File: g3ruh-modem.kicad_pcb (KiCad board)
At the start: 2 copper layers, 160 x 100 mm, 112 parts, among them P1 CONN_01X03, P2 CONN_01X06, P3 CONN_01X05, P4 C96ABC, Q1 LM7805_TO220, U1 4029, U10 LM339, U11 74HC14, U12 74HC164, U13 74HC86, U14 74HC164, U15 27C128, U16 TL084, U17 74HC74, U18 74HC164, U19 ZN429E-8, U2 27C128, U3 4029, U4 74HC164, U5 74HC74, U6 74HC86, U7 74HC164, U8 74HC161, U9 ZN429E-8

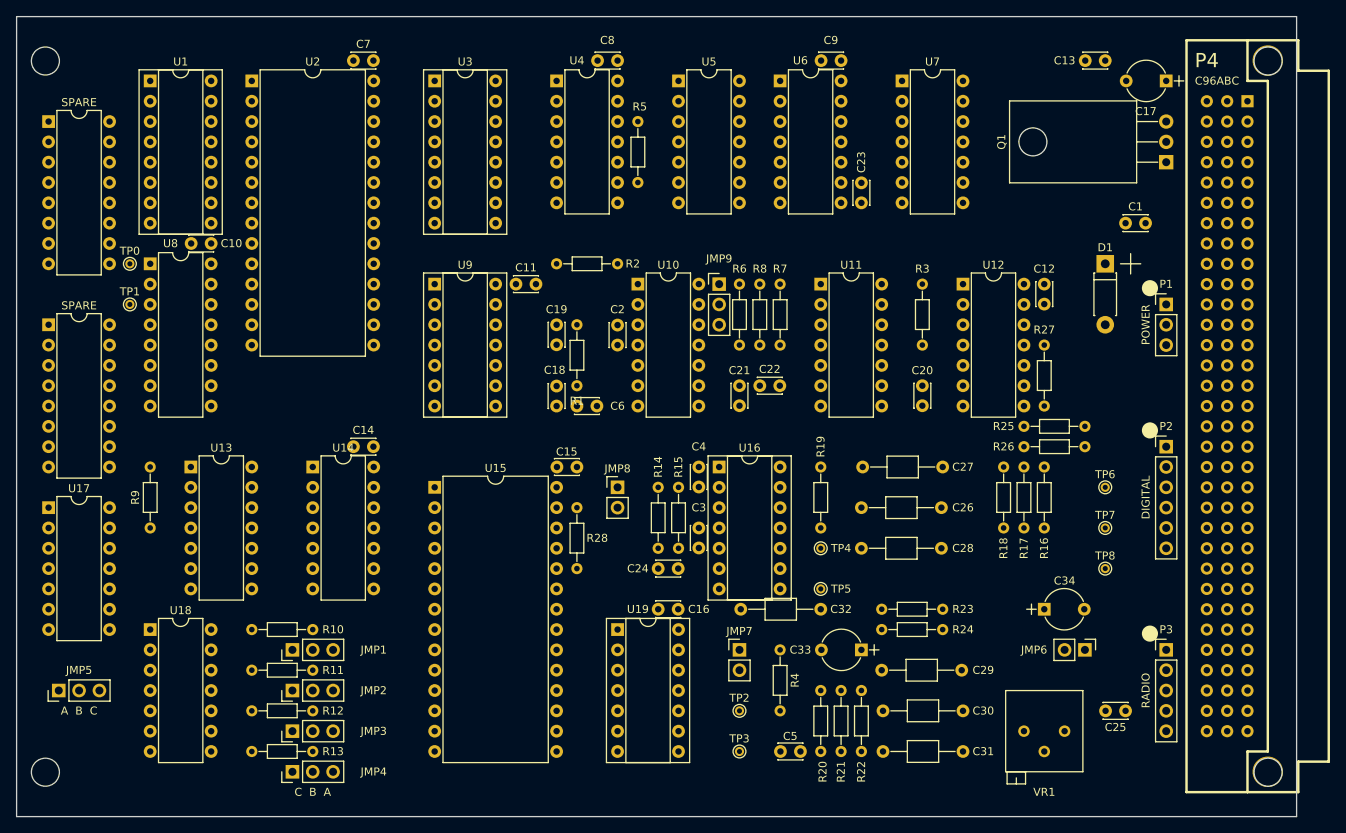
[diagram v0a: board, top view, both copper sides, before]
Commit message: Completed routing.
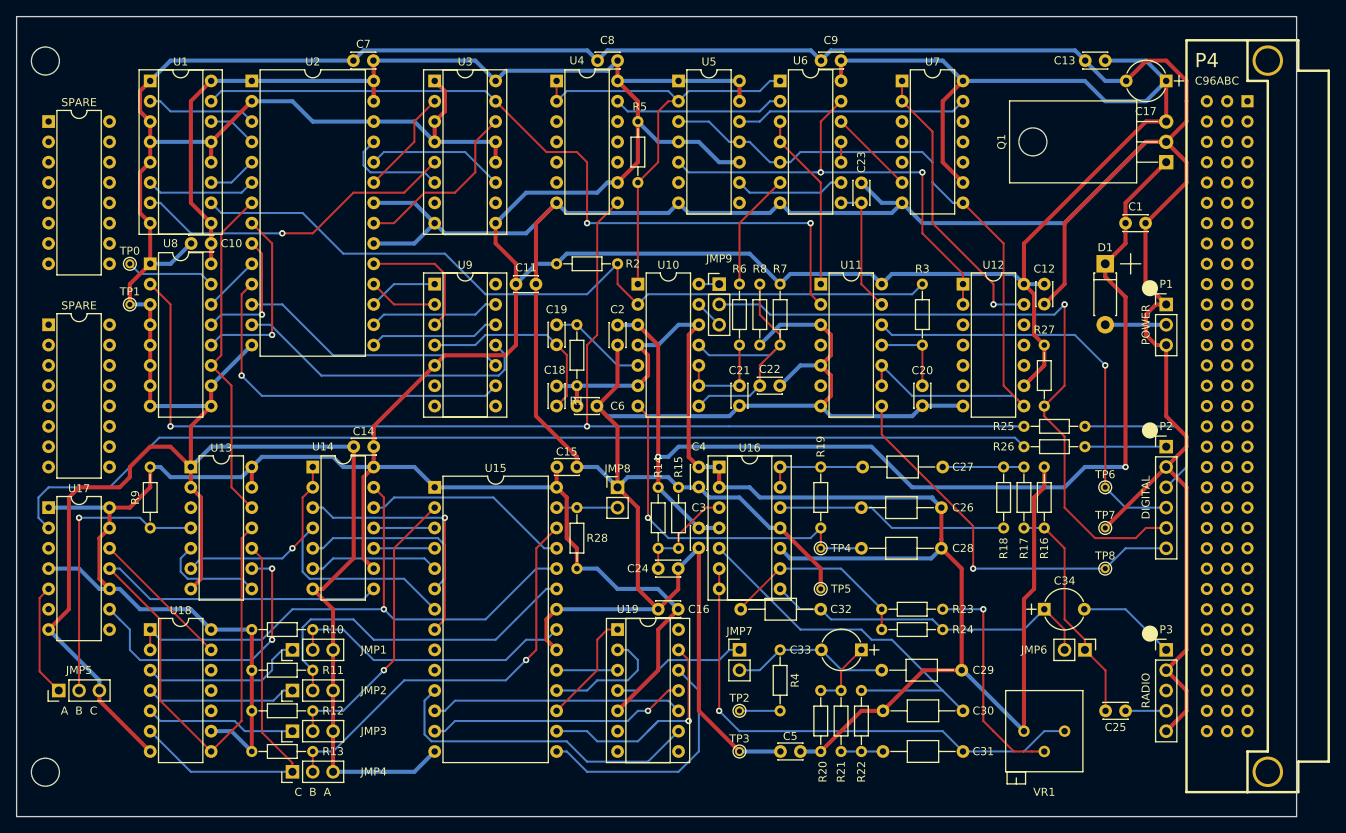
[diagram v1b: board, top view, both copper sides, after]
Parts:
- removed the REF** at (229.6, 137.8)
- removed the REF** at (229.6, 48.9)
- moved C14 2.54 mm to (117.8, 97.1), turned to 180 degrees
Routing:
- net GND: track 0.00 -> 940.6 mm
- net +5V: track 0.00 -> 575.9 mm
- net VREF: track 0.00 -> 192.3 mm
- net /ZERO CROSSING/TX_CLOCK: track 0.00 -> 155.0 mm, vias 0 -> 2
- net +12V: track 0.00 -> 138.1 mm, vias 0 -> 2
- net Net-(R26-Pad1): track 0.00 -> 131.1 mm
- net Net-(R2-Pad2): track 0.00 -> 99.9 mm
- net Net-(U1-Pad15): track 0.00 -> 97.4 mm, vias 0 -> 2
- net /LOCK_DETECT/~RX_CLOCK: track 0.00 -> 93.3 mm
- net Net-(U13-Pad11): track 0.00 -> 93.3 mm
- net DCD: track 0.00 -> 86.5 mm, vias 0 -> 1
- net Net-(U14-Pad13): track 0.00 -> 74.4 mm, vias 0 -> 1
- net Net-(C31-Pad1): track 0.00 -> 64.1 mm, vias 0 -> 1
- net Net-(U12-Pad1): track 0.00 -> 59.6 mm, vias 0 -> 2
- net /UNSCRAMBLER/RX_FILTER: track 0.00 -> 58.3 mm
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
